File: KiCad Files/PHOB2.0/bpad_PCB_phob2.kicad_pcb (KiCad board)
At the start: 2 copper layers, 31.6 x 54.4 mm, 29 parts, among them J1 Conn_01x06, SW1 C_left, SW2 C_up, SW3 C_down, SW4 C_right, U1 MCP3202

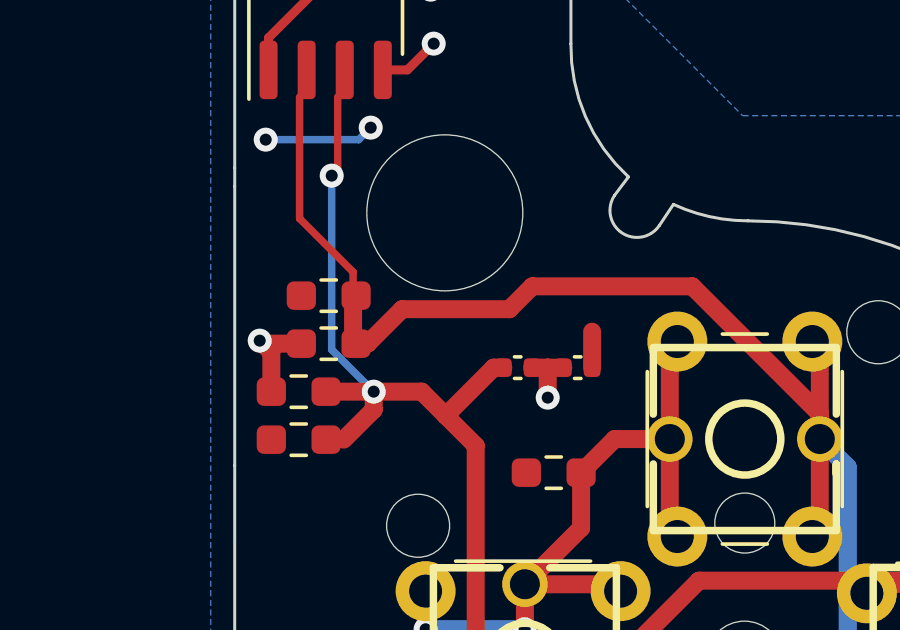
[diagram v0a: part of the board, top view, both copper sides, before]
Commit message: Fix
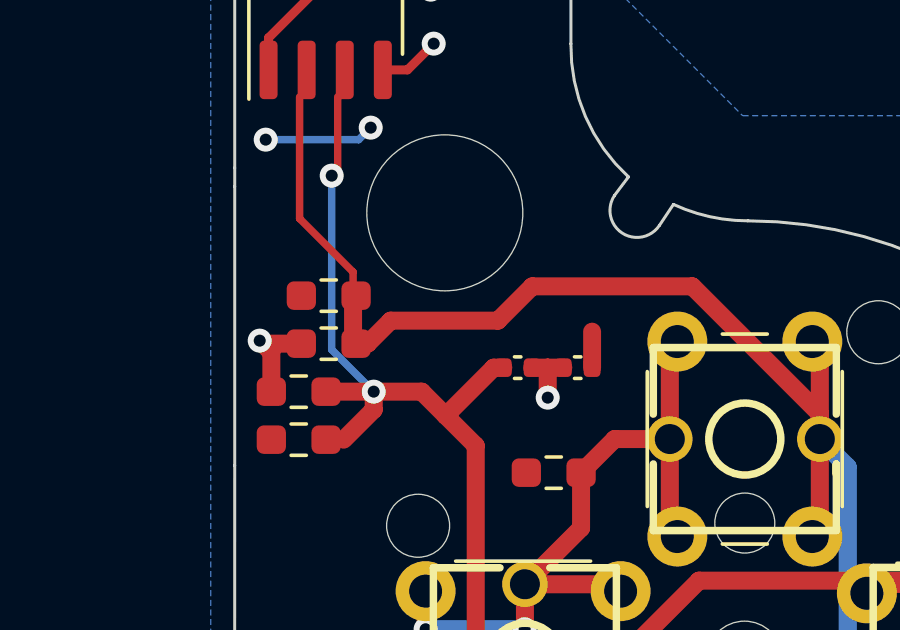
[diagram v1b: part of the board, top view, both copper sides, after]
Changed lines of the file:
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@@
   (segment (start 122.6 99.9) (end 122.6 94.1) (width 0.25) (layer "B.Cu") (net 2))
   (segment (start 124 101.3) (end 122.6 99.9) (width 0.25) (layer "B.Cu") (net 2))
-  (segment (start 128.524 98.552) (end 124.948 98.552) (width 0.6) (layer "F.Cu") (net 3))
+  (segment (start 124.567 98.933) (end 123.8 99.7) (width 0.6) (layer "F.Cu") (net 3))
   (segment (start 138.87 102.04) (end 134.62 97.79) (width 0.6) (layer "F.Cu") (net 3))
-  (segment (start 134.62 97.79) (end 129.286 97.79) (width 0.6) (layer "F.Cu") (net 3))
   (segment (start 123.4125 98.1) (end 123.3125 98.2) (width 0.6) (layer "F.Cu") (net 3))
   (segment (start 138.87 102.88) (end 138.87 99.88) (width 0.6) (layer "F.Cu") (net 3))
-  (segment (start 124.948 98.552) (end 123.8 99.7) (width 0.6) (layer "F.Cu") (net 3))
+  (segment (start 134.62 97.79) (end 129.286 97.79) (width 0.6) (layer "F.Cu") (net 3))
   (segment (start 133.87 117.54) (end 133.87 114.54) (width 0.6) (layer "F.Cu") (net 3))
+  (segment (start 138.87 102.88) (end 138.87 102.04) (width 0.6) (layer "F.Cu") (net 3))
   (segment (start 133.87 114.54) (end 134.12 114.29) (width 0.6) (layer "F.Cu") (net 3))
   (segment (start 121.53 91.475) (end 121.53 95.53) (width 0.25) (layer "F.Cu") (net 3))
   (segment (start 138.87 99.88) (end 138.62 99.63) (width 0.6) (layer "F.Cu") (net 3))
   (segment (start 138.87 102.88) (end 138.87 105.88) (width 0.6) (layer "F.Cu") (net 3))
-  (segment (start 123.8 99.7) (end 123.4125 99.7) (width 0.6) (layer "F.Cu") (net 3))
+  (segment (start 129.286 97.79) (end 128.143 98.933) (width 0.6) (layer "F.Cu") (net 3))
+  (segment (start 128.143 98.933) (end 124.567 98.933) (width 0.6) (layer "F.Cu") (net 3))
   (segment (start 133.87 120.54) (end 134.12 120.79) (width 0.6) (layer "F.Cu") (net 3))
   (segment (start 131.28 100.5) (end 131.28 99.3) (width 0.6) (layer "F.Cu") (net 3))
   (segment (start 123.3125 98.2) (end 123.3125 99.7) (width 0.6) (layer "F.Cu") (net 3))
   (segment (start 121.53 95.53) (end 123.3125 97.3125) (width 0.25) (layer "F.Cu") (net 3))
-  (segment (start 129.286 97.79) (end 128.524 98.552) (width 0.6) (layer "F.Cu") (net 3))
   (segment (start 138.87 105.88) (end 138.62 106.13) (width 0.6) (layer "F.Cu") (net 3))
-  (segment (start 138.87 102.88) (end 138.87 102.04) (width 0.6) (layer "F.Cu") (net 3))
   (segment (start 123.3125 97.3125) (end 123.3125 98.1) (width 0.25) (layer "F.Cu") (net 3))
   (segment (start 133.87 117.54) (end 133.87 120.54) (width 0.6) (layer "F.Cu") (net 3))
+  (segment (start 123.8 99.7) (end 123.4125 99.7) (width 0.6) (layer "F.Cu") (net 3))
   (segment (start 139.8 111.500281) (end 139.8 103.81) (width 0.6) (layer "B.Cu") (net 3))
   (segment (start 133.87 113.594491) (end 134.664491 112.8) (width 0.6) (layer "B.Cu") (net 3))

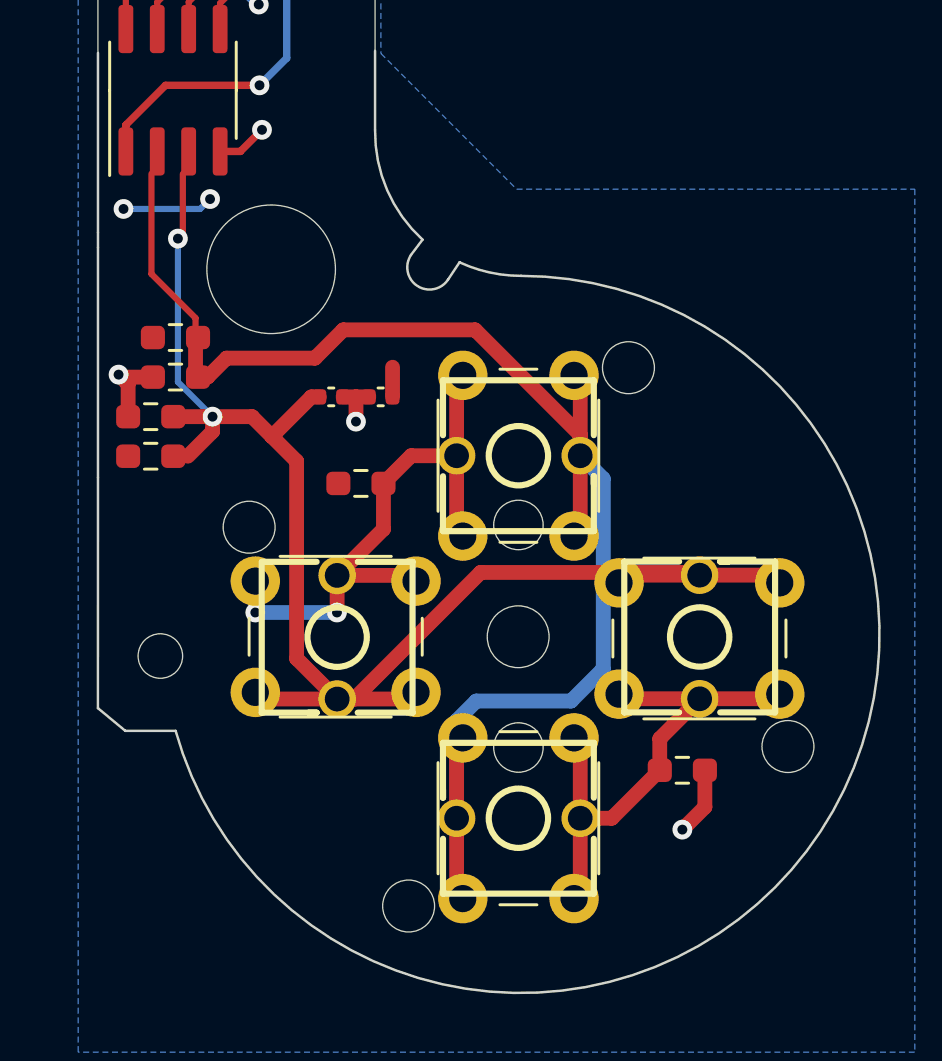
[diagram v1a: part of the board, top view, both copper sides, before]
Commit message: cleaned up and fixed
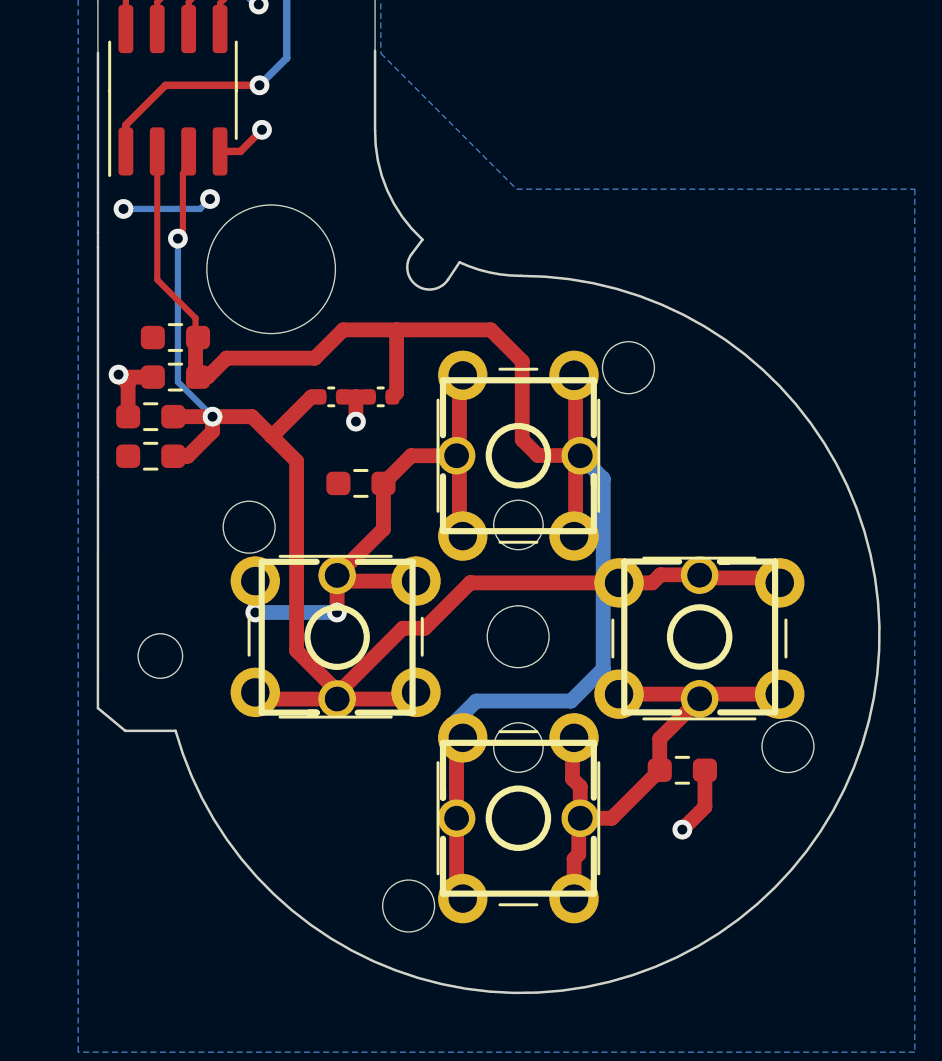
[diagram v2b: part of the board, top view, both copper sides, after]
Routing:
- net /C_x: track 62.2 -> 66.0 mm
- net /C_y: track 62.0 -> 60.1 mm
- net Net-(SW2-Pad1): track 23.6 -> 24.3 mm

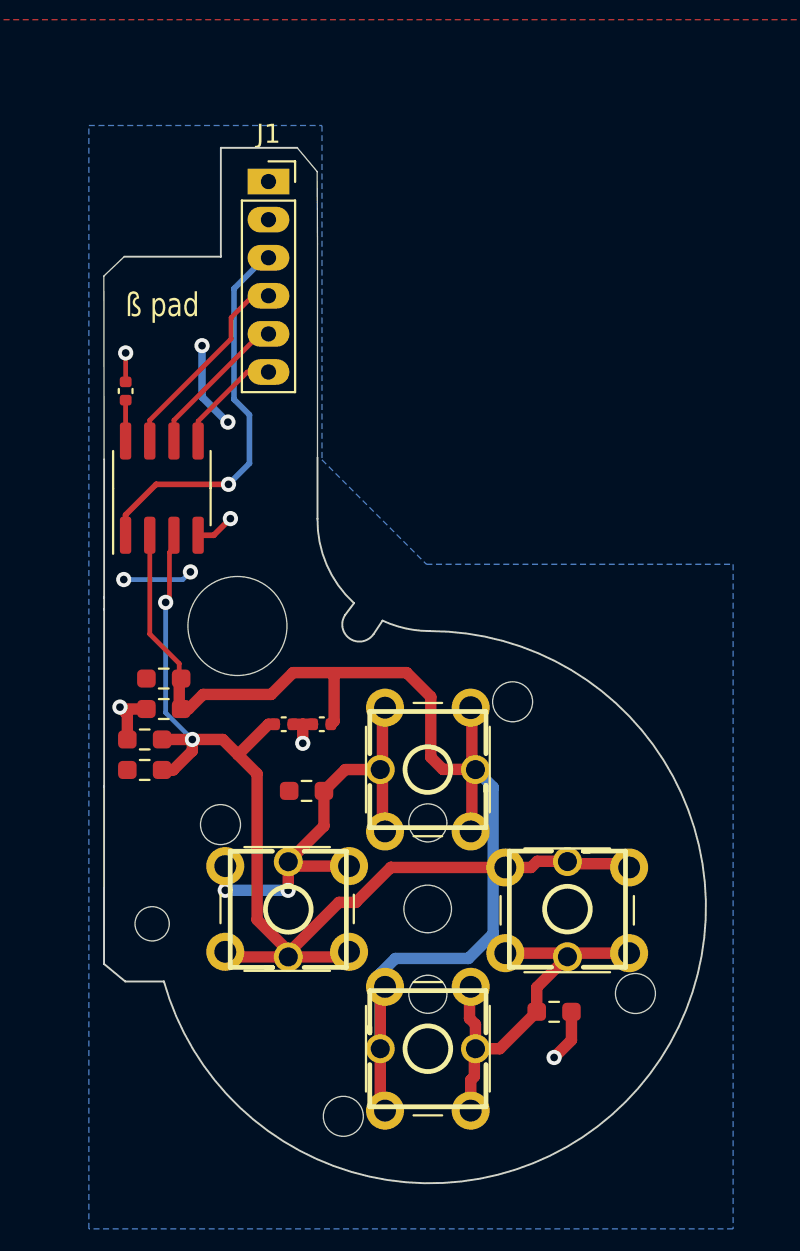
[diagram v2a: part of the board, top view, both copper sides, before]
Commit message: New PC
Untested
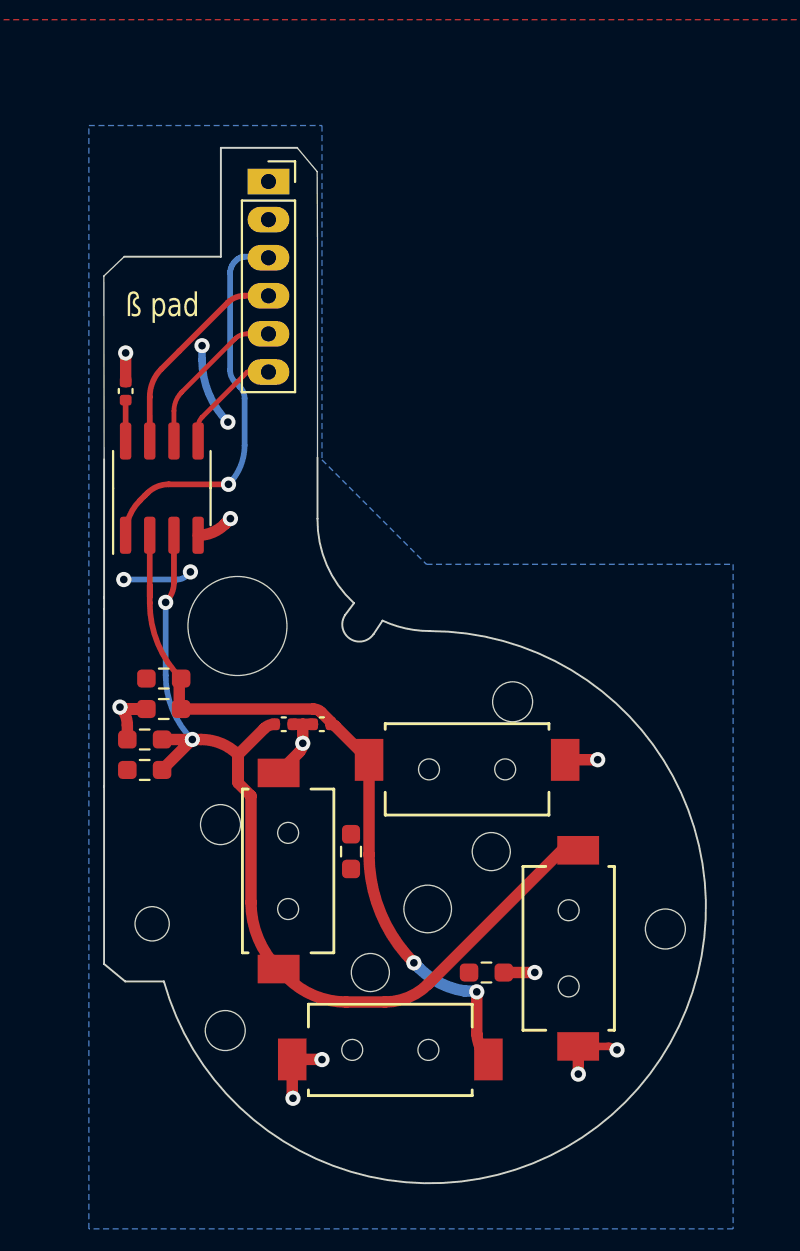
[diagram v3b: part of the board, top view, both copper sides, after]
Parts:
- removed the REF** at (146.9, 112.5)
- removed the REF** at (138.6, 114.3)
- removed the REF** at (125.7, 108.0)
- removed the REF** at (134.1, 106.1)
- removed SW1: C_left, easyeda2kicad:SW-TH_L6.2-W6.2-P5.00
- removed SW2: C_up, easyeda2kicad:SW-TH_L6.2-W6.2-P5.00
- removed SW3: C_down, easyeda2kicad:SW-TH_L6.2-W6.2-P5.00
- removed SW4: C_right, easyeda2kicad:SW-TH_L6.2-W6.2-P5.00
- added REF**: , eec:Omron-D2LS-11-0, F.Cu at (134.4, 117.6)
- added REF**: , eec:Omron-D2LS-11-0, F.Cu at (138.4, 102.9)
- added REF**: , eec:Omron-D2LS-11-0, F.Cu at (129.0, 108.2)
- added REF**: , eec:Omron-D2LS-11-0, F.Cu at (143.8, 112.3)
- moved H4 7.66 mm to (125.7, 116.6)
- moved R1 4.11 mm to (139.4, 113.5)
- moved R2 3.95 mm to (132.3, 107.2), turned to -90 degrees
- moved H3 3.74 mm to (148.8, 111.3)
- moved H13 3.66 mm to (139.7, 107.2)
- moved H12 3.23 mm to (133.3, 113.5)
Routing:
- net /C_x: track 66.0 -> 39.9 mm, vias 0 -> 2
- net Net-(SW2-Pad1): track 24.3 -> 0.00 mm, vias 2 -> 0
- net Net-(R1-Pad1): track 21.3 -> 0.00 mm
- net GND: track 11.6 -> 25.8 mm, vias 5 -> 10
- net /C_y: track 60.1 -> 52.9 mm
- net /CLK2: track 11.4 -> 13.2 mm
- net /Dout2: track 7.95 -> 9.28 mm
